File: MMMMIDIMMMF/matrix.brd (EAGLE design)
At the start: 30 x 70 mm, 10 parts

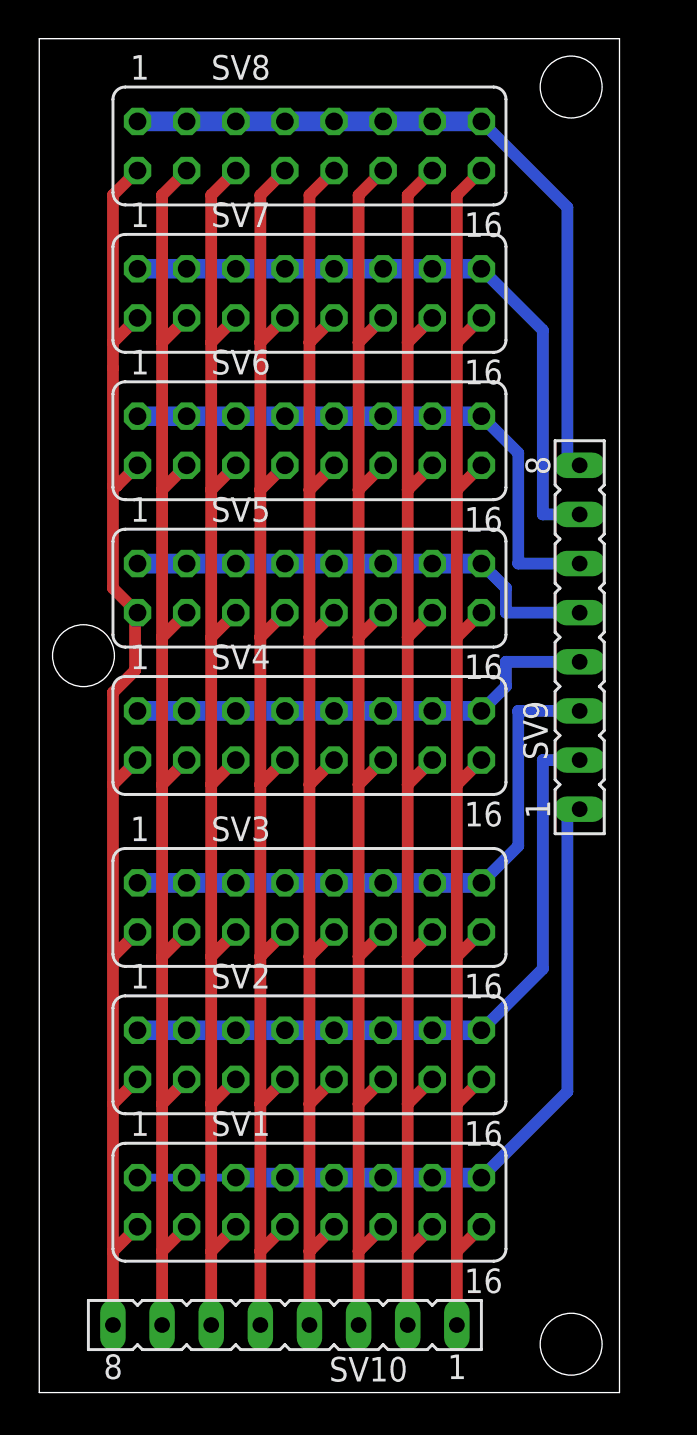
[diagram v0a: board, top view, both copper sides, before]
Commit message: Matrix board
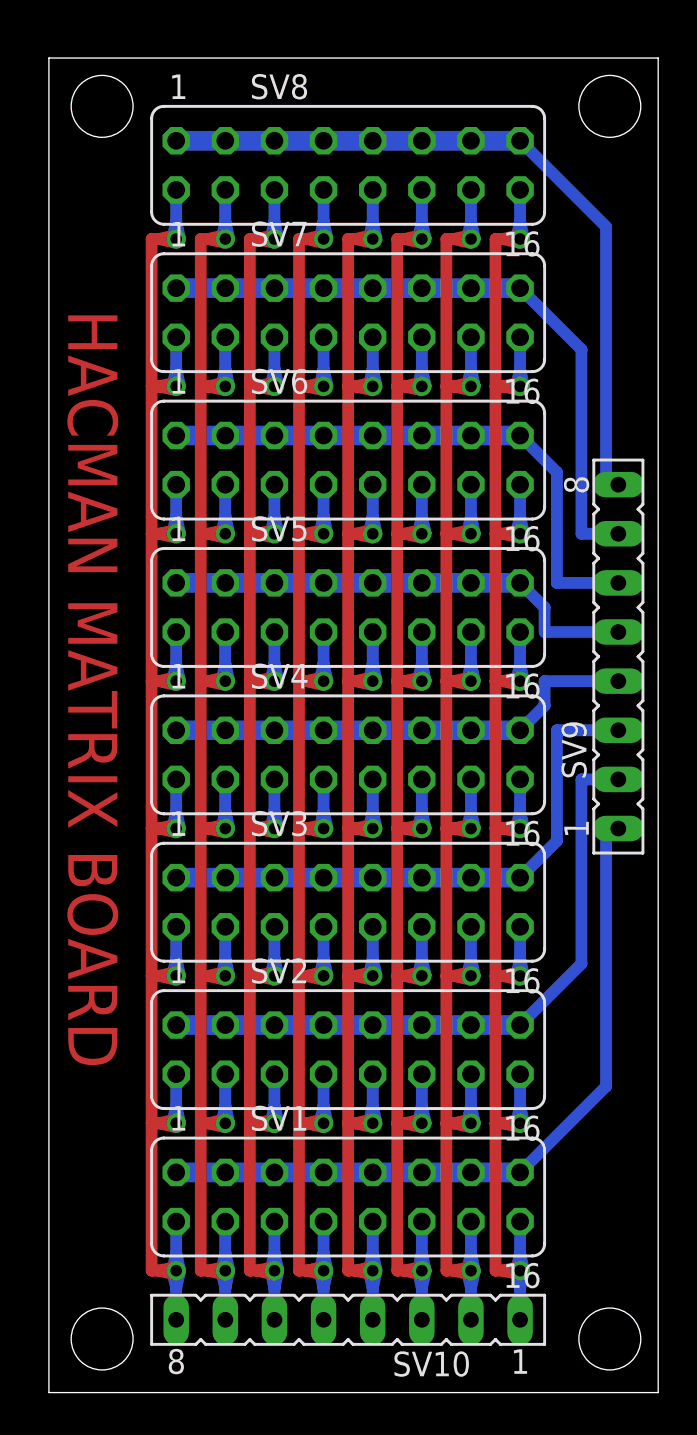
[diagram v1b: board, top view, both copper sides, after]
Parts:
- moved SV10 3.28 mm to (16.0, 3.76)
- moved SV4 2.24 mm to (16.0, 33.0)
- moved SV5 2.24 mm to (16.0, 40.6)
- moved SV6 2.24 mm to (16.0, 48.2)
- moved SV7 2.24 mm to (16.0, 55.8)
- moved SV8 2.24 mm to (16.0, 63.5)
- moved SV9 2.24 mm to (29.9, 38.1)
- moved SV1 2.02 mm to (16.0, 10.1)
- moved SV2 2.02 mm to (16.0, 17.7)
- moved SV3 2.02 mm to (16.0, 25.4)
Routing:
- net C8: track 72.0 -> 123.0 mm, vias 0 -> 8
- net C7: track 72.8 -> 123.0 mm, vias 0 -> 8
- net C5: track 72.8 -> 123.0 mm, vias 0 -> 8
- net C4: track 72.8 -> 123.0 mm, vias 0 -> 8
- net C6: track 72.8 -> 123.0 mm, vias 0 -> 8
- net C3: track 72.8 -> 123.0 mm, vias 0 -> 8
- net C2: track 72.8 -> 123.0 mm, vias 0 -> 8
- net C1: track 72.8 -> 123.0 mm, vias 0 -> 8
- net N$3: track 30.6 -> 29.4 mm
- net N$2: track 35.0 -> 33.7 mm
- net N$1: track 39.3 -> 38.0 mm
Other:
- board size 30 x 70 mm -> 31.5 x 69 mm
- board text added: "HACMAN MATRIX BOARD"
